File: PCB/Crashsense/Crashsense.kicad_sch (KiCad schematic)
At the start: 49 parts, among them J1 u-blox NEO-M8N, J2 Micro_SD_Card_Det1, J3 BATTERY_CONNECTOR, J4 Debug_pins, J5 Coincell_BAT, P1 USB_C_Plug_USB2.0, SW1 SW_Push, SW2 SW_Push, U1 ESP32-S3-WROOM-1, U2 ADXL377, U3 BMM150, U4 DS3231M, U5 BMI270, U6 TP4056-42-ESOP8, U7 ME6211C10M5

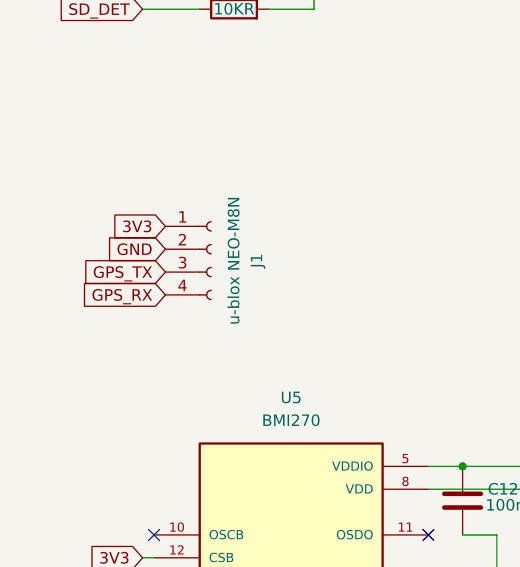
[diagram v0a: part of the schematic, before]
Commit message: updated things
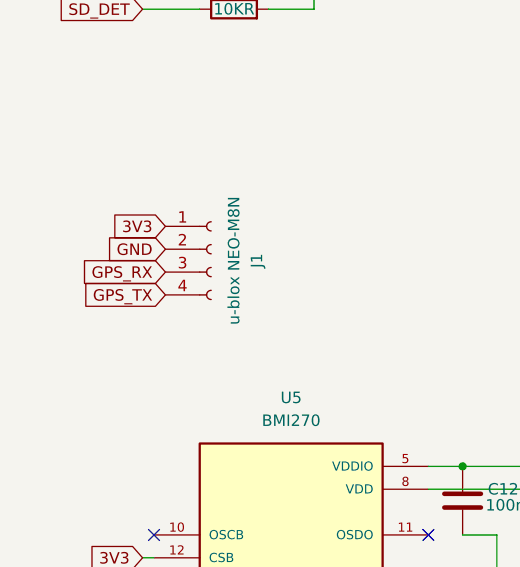
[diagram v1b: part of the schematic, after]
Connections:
- net GPS_RX: now also J1.3 (Pin_3); no longer J1.4 (Pin_4)
- net GPS_TX: now also J1.4 (Pin_4); no longer J1.3 (Pin_3)
